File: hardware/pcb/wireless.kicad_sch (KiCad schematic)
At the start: 36 parts, among them IC2 MAYA-W386-00B, Y3 32kHz768

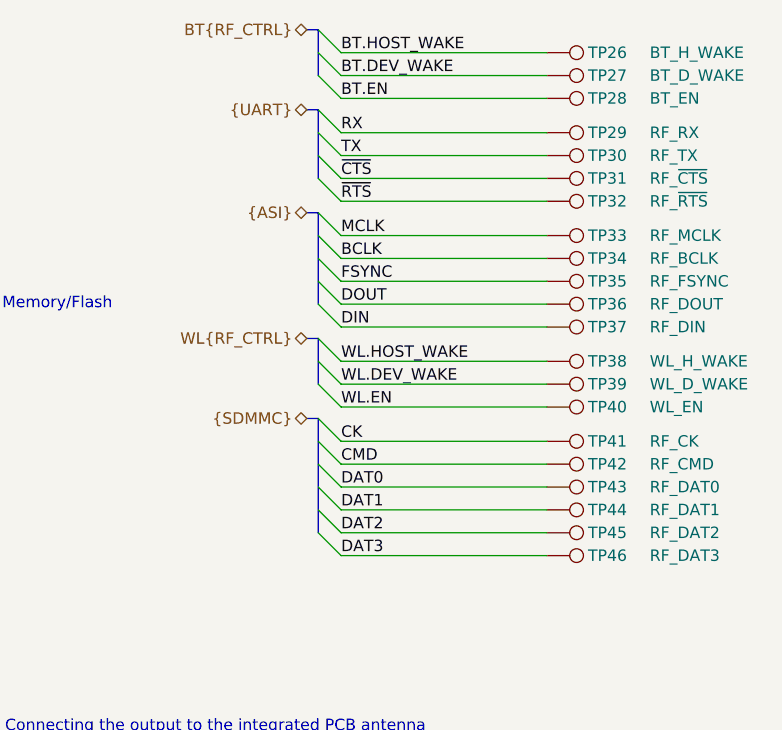
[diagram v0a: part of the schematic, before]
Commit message: cleanup, tespoints, passives
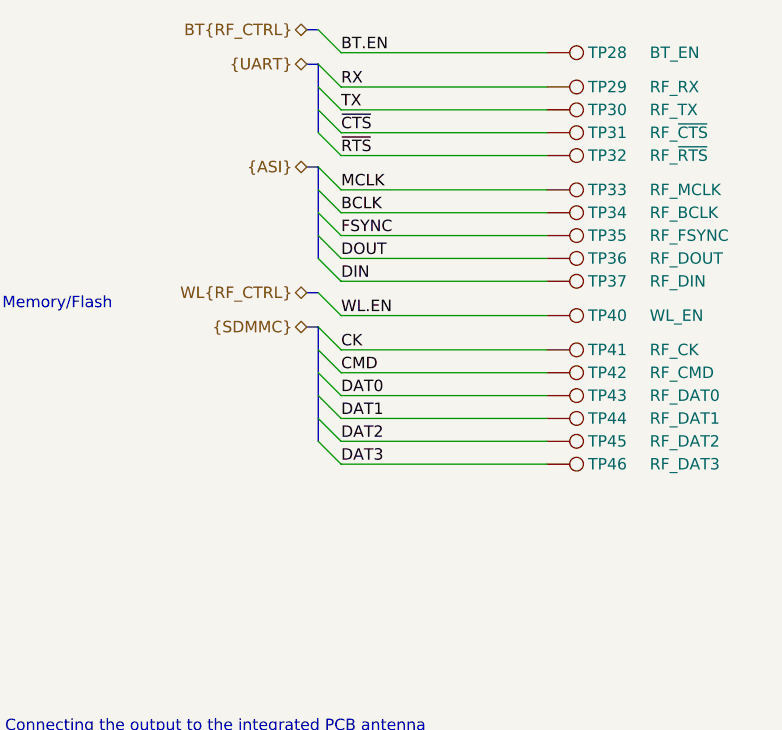
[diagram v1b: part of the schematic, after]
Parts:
- removed TP26: BT_H_WAKE, TestPoint:TestPoint_Pad_D1.0mm, symbol Connector:TestPoint
- removed TP27: BT_D_WAKE, TestPoint:TestPoint_Pad_D1.0mm, symbol Connector:TestPoint
- removed TP38: WL_H_WAKE, TestPoint:TestPoint_Pad_D1.0mm, symbol Connector:TestPoint
- removed TP39: WL_D_WAKE, TestPoint:TestPoint_Pad_D1.0mm, symbol Connector:TestPoint
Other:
- moved on the sheet: TP28, TP29, TP30, TP31, TP32, TP33, TP34, TP35, TP36, TP37, TP40, TP41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
